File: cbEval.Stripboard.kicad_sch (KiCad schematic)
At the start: 33 parts, among them J1 Bergstik-II_3, J10 Socket.Hor.2x5.6-5535512-4, J11 Bergstik-II_3, J12 Bergstik-II_3, J13 Bergstik-II_6, J14 Bergstik-II_8, J15 Bergstik-II_6, J2 Bergstik-II_6, J3 Keystone.4918, J4 Keystone.4918, J5 Keystone.3571, J6 Keystone.3571, J7 Socket.Hor.2x5.6-5535512-4, J8 Header.Hor.2x5.9-103326-0-05, J9 Header.Hor.2x5.9-103326-0-05, U1 SN74AHC138D

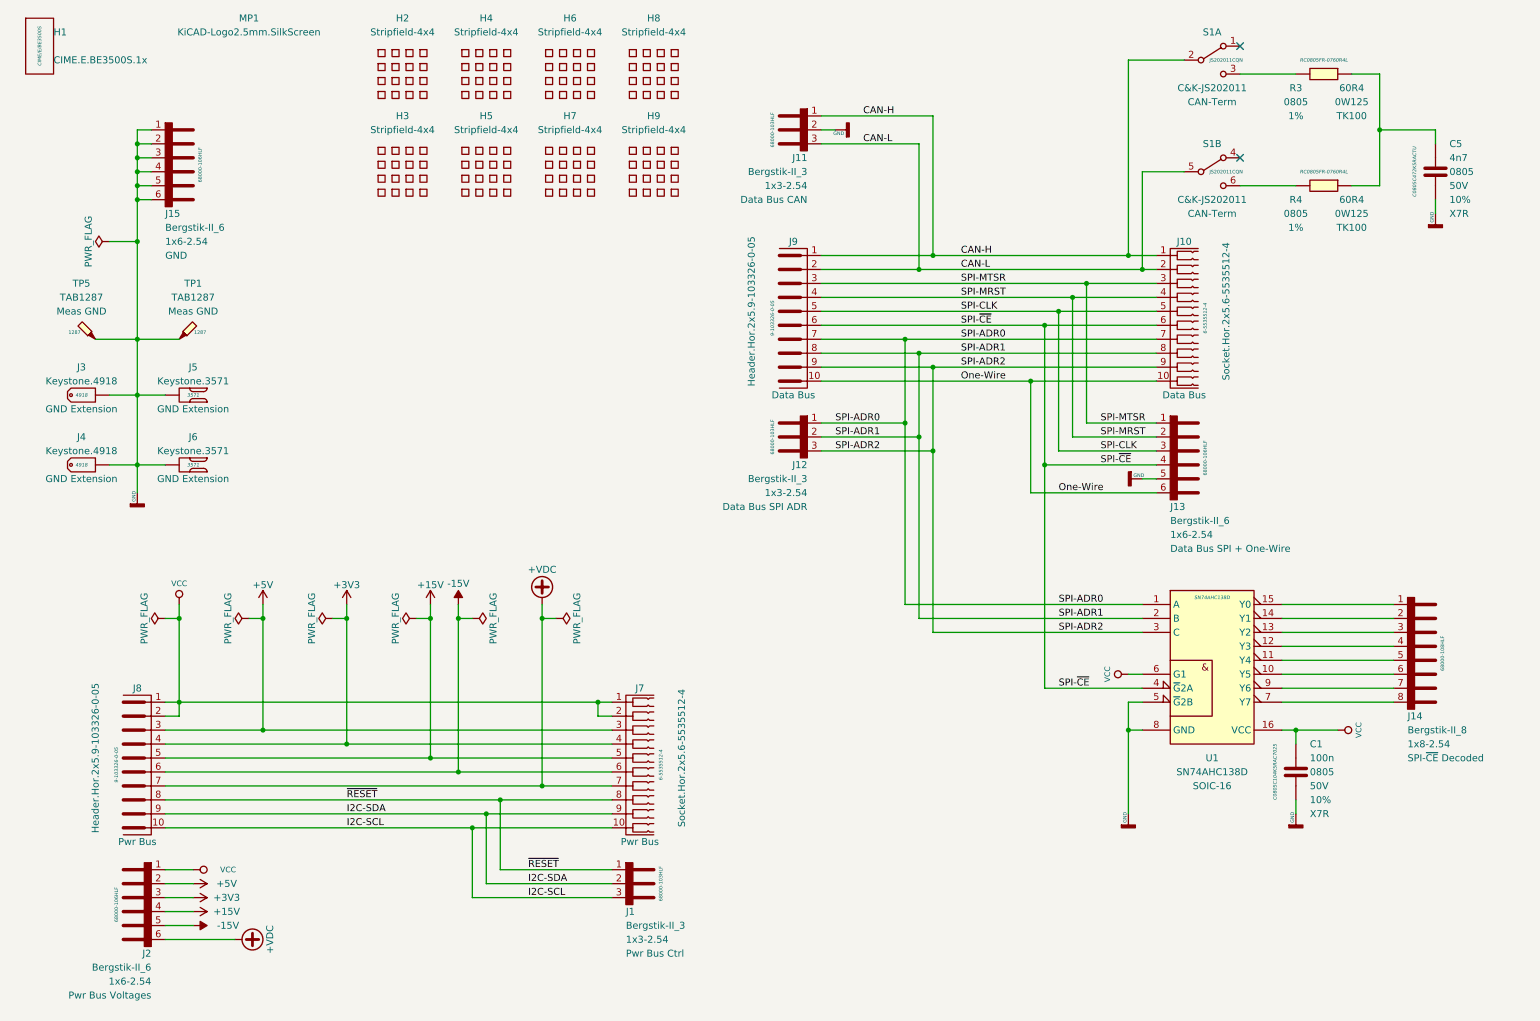
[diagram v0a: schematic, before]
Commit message: Bus-Stecker getauscht, BOM erstellt
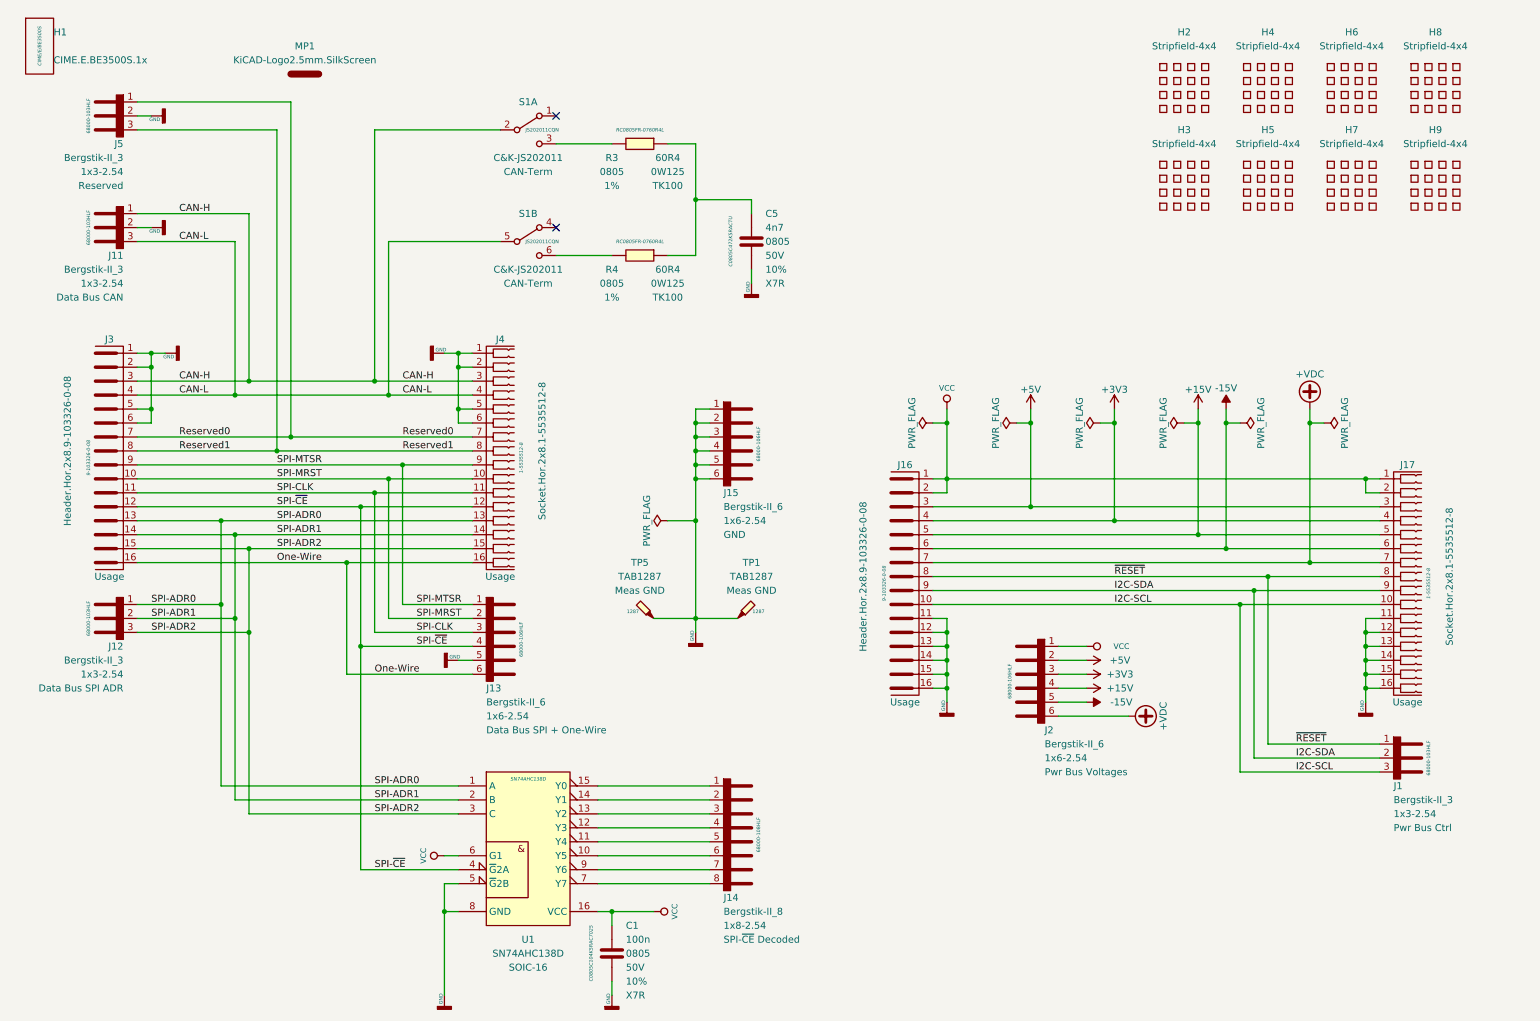
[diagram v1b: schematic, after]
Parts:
- removed J10, J7: Socket.Hor.2x5.6-5535512-4, BTech.Connector.AMPMODU-ModII:Socket.Hor.2x5.6-5535512-4, symbol J.AMPMODU-ModII:Socket.Hor.2x5.6-5535512-4
- removed J3, J4: Keystone.4918, BTech.Connector.QuickConnect:Keystone.4918, symbol J.QuickConnect:Keystone.4918
- removed J5, J6: Keystone.3571, BTech.Connector.QuickConnect:Keystone.3571, symbol J.QuickConnect:Keystone.3571
- removed J8, J9: Header.Hor.2x5.9-103326-0-05, Connector_PinHeader_2.54mm:PinHeader_2x05_P2.54mm_Horizontal, symbol J.AMPMODU-ModII:Header.Hor.2x5.9-103326-0-05
- added J16, J3: Header.Hor.2x8.9-103326-0-08, Connector_PinHeader_2.54mm:PinHeader_2x08_P2.54mm_Horizontal, symbol J.AMPMODU-ModII:Header.Hor.2x8.9-103326-0-08
- added J17, J4: Socket.Hor.2x8.1-5535512-8, BTech.Connector.AMPMODU-ModII:Socket.Hor.2x5.6-5535512-4, symbol J.AMPMODU-ModII:Socket.Hor.2x8.1-5535512-8
- added J5: Bergstik-II_3, Connector_PinHeader_2.54mm:PinHeader_1x03_P2.54mm_Vertical, symbol J.PinHeader:Bergstik-II_3
- MP1: footprint Symbol:KiCad-Logo2_5mm_SilkScreen -> Symbol:KiCad-Logo_5mm_SilkScreen
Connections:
- net +15V: now also J16.5, J17.5
- net +3V3: now also J16.4, J17.4
- net +5V: now also J16.3, J17.3
- net +VDC: now also J16.7, J17.7
- net -15V: now also J16.6, J17.6
- net CAN-H: now also J3.3, J4.3
- net CAN-L: now also J3.4, J4.4
- net GND: now also J16.11, J16.12, J16.13, J16.14, J16.15, J16.16, J17.11, J17.12, J17.13, J17.14, J17.15, J17.16, J3.1, J3.2, J3.5, J3.6, J4.1, J4.2, J4.5, J4.6, J5.2 (A2)
- net I2C-SCL: now also J16.10, J17.10
- net I2C-SDA: now also J16.9, J17.9
- net One-Wire: now also J3.16, J4.16
- net SPI-ADR0: now also J3.13, J4.13
- net SPI-ADR1: now also J3.14, J4.14
- net SPI-ADR2: now also J3.15, J4.15
- net SPI-CLK: now also J3.11, J4.11
- net SPI-MRST: now also J3.10, J4.10
- net SPI-MTSR: now also J3.9, J4.9
- net SPI-~CE: now also J3.12, J4.12
- net VCC: now also J16.1, J16.2, J17.1, J17.2
- net ~RESET: now also J16.8, J17.8
- new net Reserved0: J3.7, J4.7, J5.1 (A1)
- new net Reserved1: J3.8, J4.8, J5.3 (A3)
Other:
- moved on the sheet: C1, C5, H2, H3, H4, H5, H6, H7, H8, H9, J1, J11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
